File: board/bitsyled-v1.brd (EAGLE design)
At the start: 17 x 17 mm, 8 parts

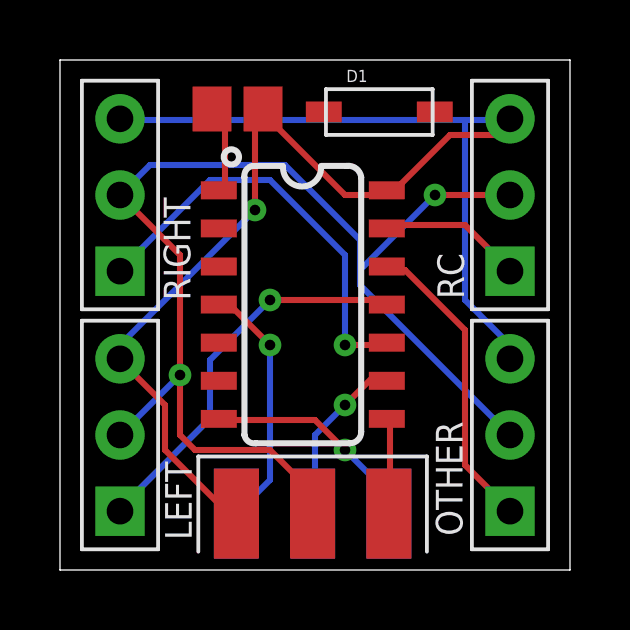
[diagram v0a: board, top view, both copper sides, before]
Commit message: Updatez
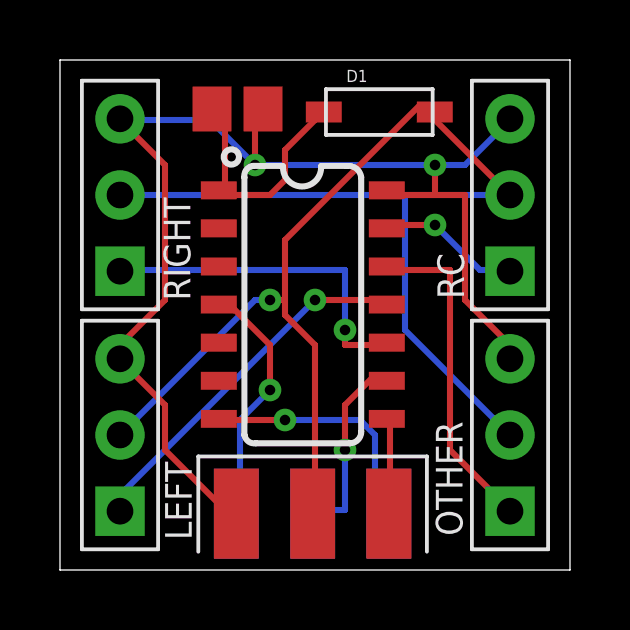
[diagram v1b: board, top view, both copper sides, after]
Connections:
- removed net VCC: D1.A
- net 5V: now also D1.A
- net VR: now also D1.C
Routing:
- net 5V: track 41.8 -> 50.1 mm, vias 2 -> 1
- net GND: track 49.5 -> 42.2 mm, vias 1 -> 2
- net VR: track 3.33 -> 8.34 mm
- net LD2: track 14.2 -> 11.4 mm
- net SDA: track 7.51 -> 8.39 mm
- net LD0: track 10.1 -> 11.0 mm
- net LD1: track 13.0 -> 12.2 mm
- net SCL: track 5.91 -> 6.50 mm
- net RC: vias 0 -> 1
